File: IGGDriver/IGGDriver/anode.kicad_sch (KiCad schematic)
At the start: 9 parts, among them Q100 Q_NPN_BEC, Q99 Q_NPN_BEC

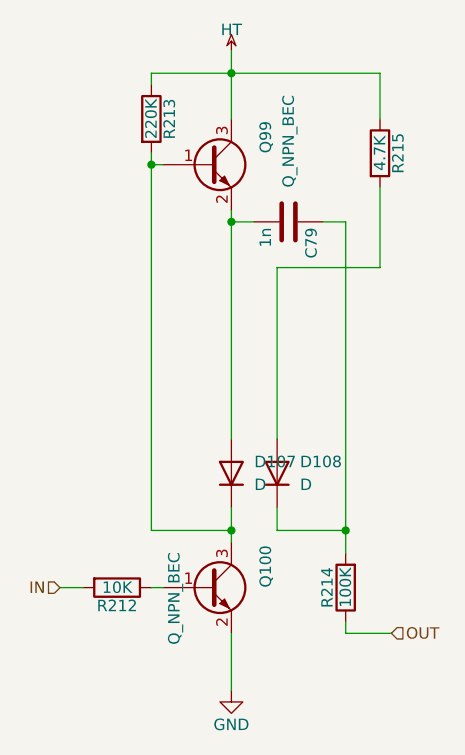
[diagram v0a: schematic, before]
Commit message: RTM
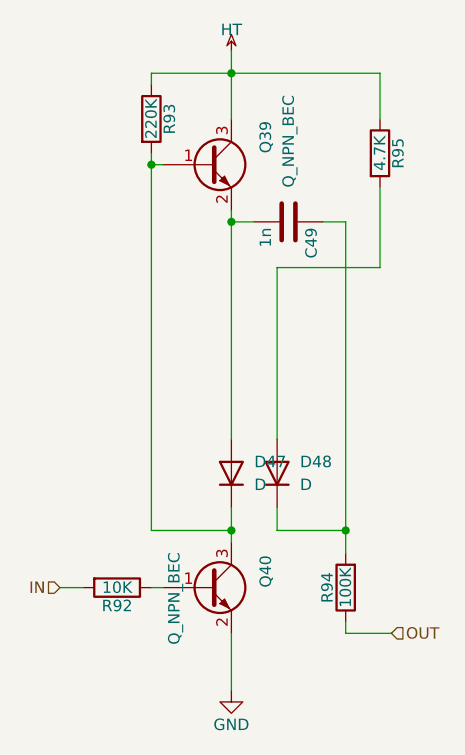
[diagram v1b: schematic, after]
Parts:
- renumbered C79 to C49, D107 to D47, D108 to D48, Q99 to Q39, Q100 to Q40, R212 to R92, R213 to R93, R214 to R94, R215 to R95
